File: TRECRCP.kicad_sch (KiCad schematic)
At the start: 16 parts, among them SW1 Dispatch2, SW1 Key On/Off Switch, SW2 Maintenince Rotary Switch, SW4 Restart, SW5 Dispatch1, SW8 Stop

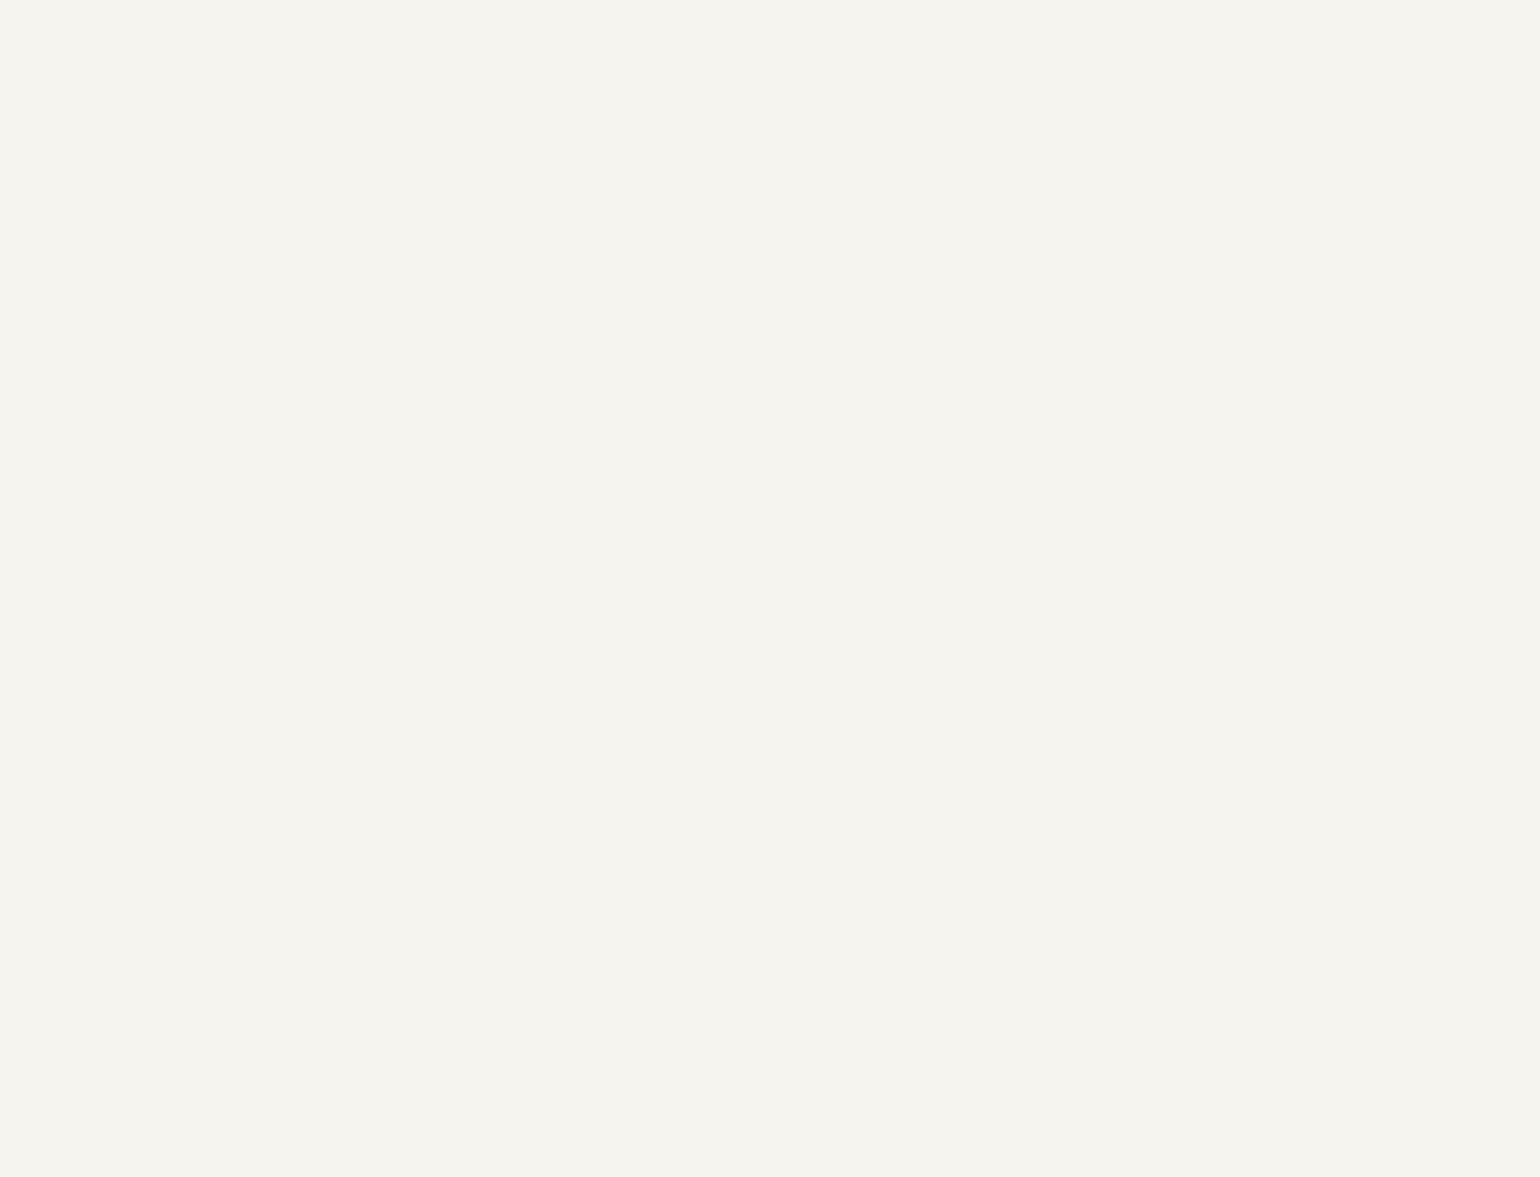
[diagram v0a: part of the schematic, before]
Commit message: wip
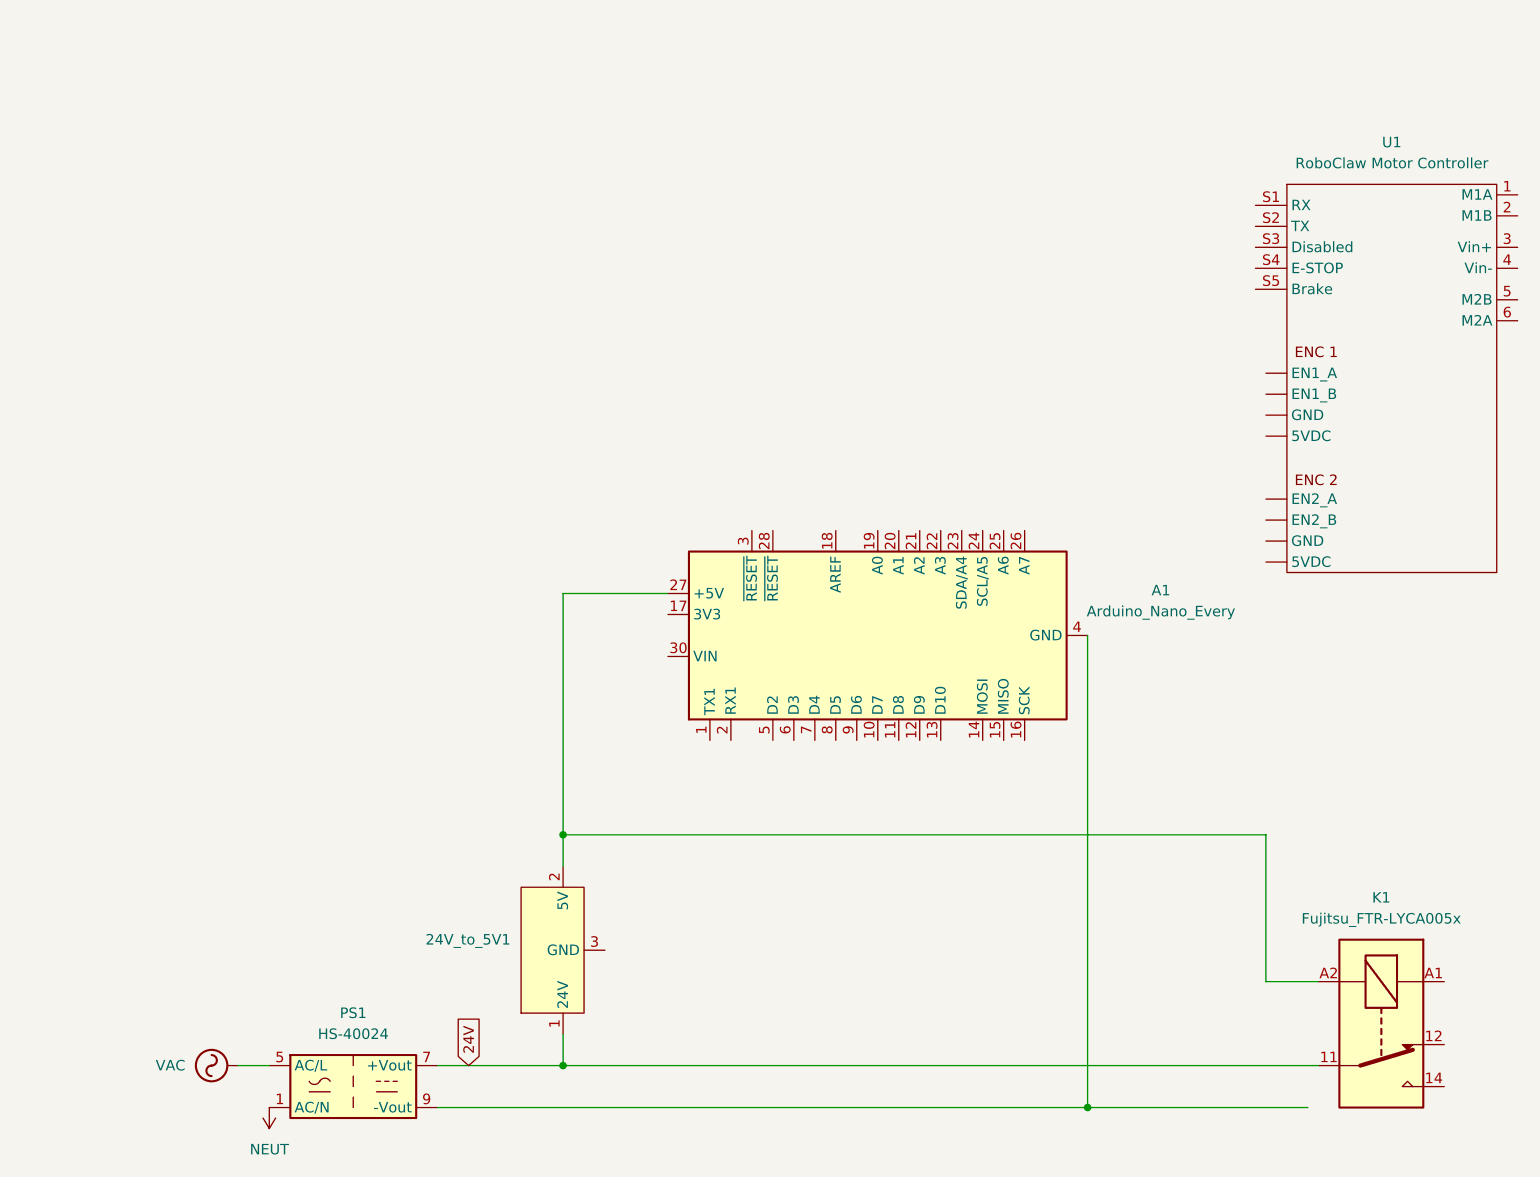
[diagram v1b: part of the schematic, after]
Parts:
- added 24V_to_5V1: ~, symbol TREC SYMBOL LIB:24v_-{gt}_5v
- added A1: Arduino_Nano_Every, Module:Arduino_Nano, symbol MCU_Module:Arduino_Nano_Every
- added K1: Fujitsu_FTR-LYCA005x, Relay_THT:Relay_SPDT_Fujitsu_FTR-LYCA005x_FormC_Vertical, symbol Relay:Fujitsu_FTR-LYCA005x
- added PS1: HS-40024, Converter_ACDC:Converter_ACDC_Hahn_HS-400xx_THT, symbol Converter_ACDC:HS-40024
- added U1: RoboClaw Motor Controller, symbol custom symbols:RoboClaw_2x30A_MC
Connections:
- new net: 24V_to_5V1.2 (5V), A1.27 (+5V), K1.A2
- new net: A1.29 (GND), A1.4 (GND), PS1.9 (-Vout)
- new net 24V: 24V_to_5V1.1 (24V), K1.11, PS1.7 (+Vout)
- new net NEUT: PS1.1 (AC/N)
- new net VAC: PS1.5 (AC/L)

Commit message: Base elec diagram
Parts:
- added U2, U3: 5304 Gear Motor, symbol custom symbols:5304_Saturn_Gear_Motor
- renumbered 24V_to_5V1 to 24V_to_12V
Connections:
- net at K1.14: now also U1.3 (Vin+)
- net GND: now reaches K1.A1
- net GND: now also 24V_to_12V.3 (GND)
- net at A1.13 (D10): now also U1.S4 (E-STOP)
- net at A1.29 (GND), A1.4 (GND), PS1.9 (-Vout): now also U1.4 (Vin-)
- net at A1.30 (VIN): now also 24V_to_12V.2 (12V)
- net at A1.5 (D2): now also K1.A2
- net at RCC1.10 (UART0_RX): now also U1.S2 (TX)
- net at RCC1.8 (UART0_TX): now also U1.S1 (RX)
- net at U1. (5VDC): now also U2.6 (Ch_B)
- net at U1.1 (M1A): now also U2.1 (M-)
- net at U1.2 (M1B): now also U2.2 (M+)
- net at U1.5 (M2B): now also U3.1 (M-)
- net at U1.6 (M2A): now also U3.2 (M+)
- new net: A1. (USB-B), RCC1. (USB)
- new net: U1. (5VDC), U3.3 (VCC)
- new net: U1. (5VDC), U3.4 (GND)
- new net: U1. (5VDC), U3.5 (Ch_A)
- new net: U1. (5VDC), U3.6 (Ch_B)
- new net: U1. (5VDC), U2.3 (VCC)
- new net: U1. (5VDC), U2.4 (GND)
- new net: U1. (5VDC), U2.5 (Ch_A)
- now unconnected: A1.27 (+5V)
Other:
- note added: "MAKE E-STOP LORE ACCURATE!!"
- note added: "MAKE VCLAMP CIRCUIT HERE :)"
- note added: "NEED TO FIGURE OUT HOW TO HAVE ARDUINO SWITCH RELAY!!"
- moved on the sheet: 24V_to_12V, ESTOP, K1, PS1, SW1, SW2, U1
